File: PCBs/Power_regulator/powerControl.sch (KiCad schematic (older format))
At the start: 13 parts, among them J1 Conn_01x03_Female, J2 Conn_01x06_Female, J3 Conn_01x04_Male, J4 Conn_01x01_Male, J5 Conn_01x01_Male, J6 Conn_01x01_Male, J7 Conn_01x01_Male, J8 Conn_01x03_Female, J9 Conn_01x04_Female, U1 MAX9938

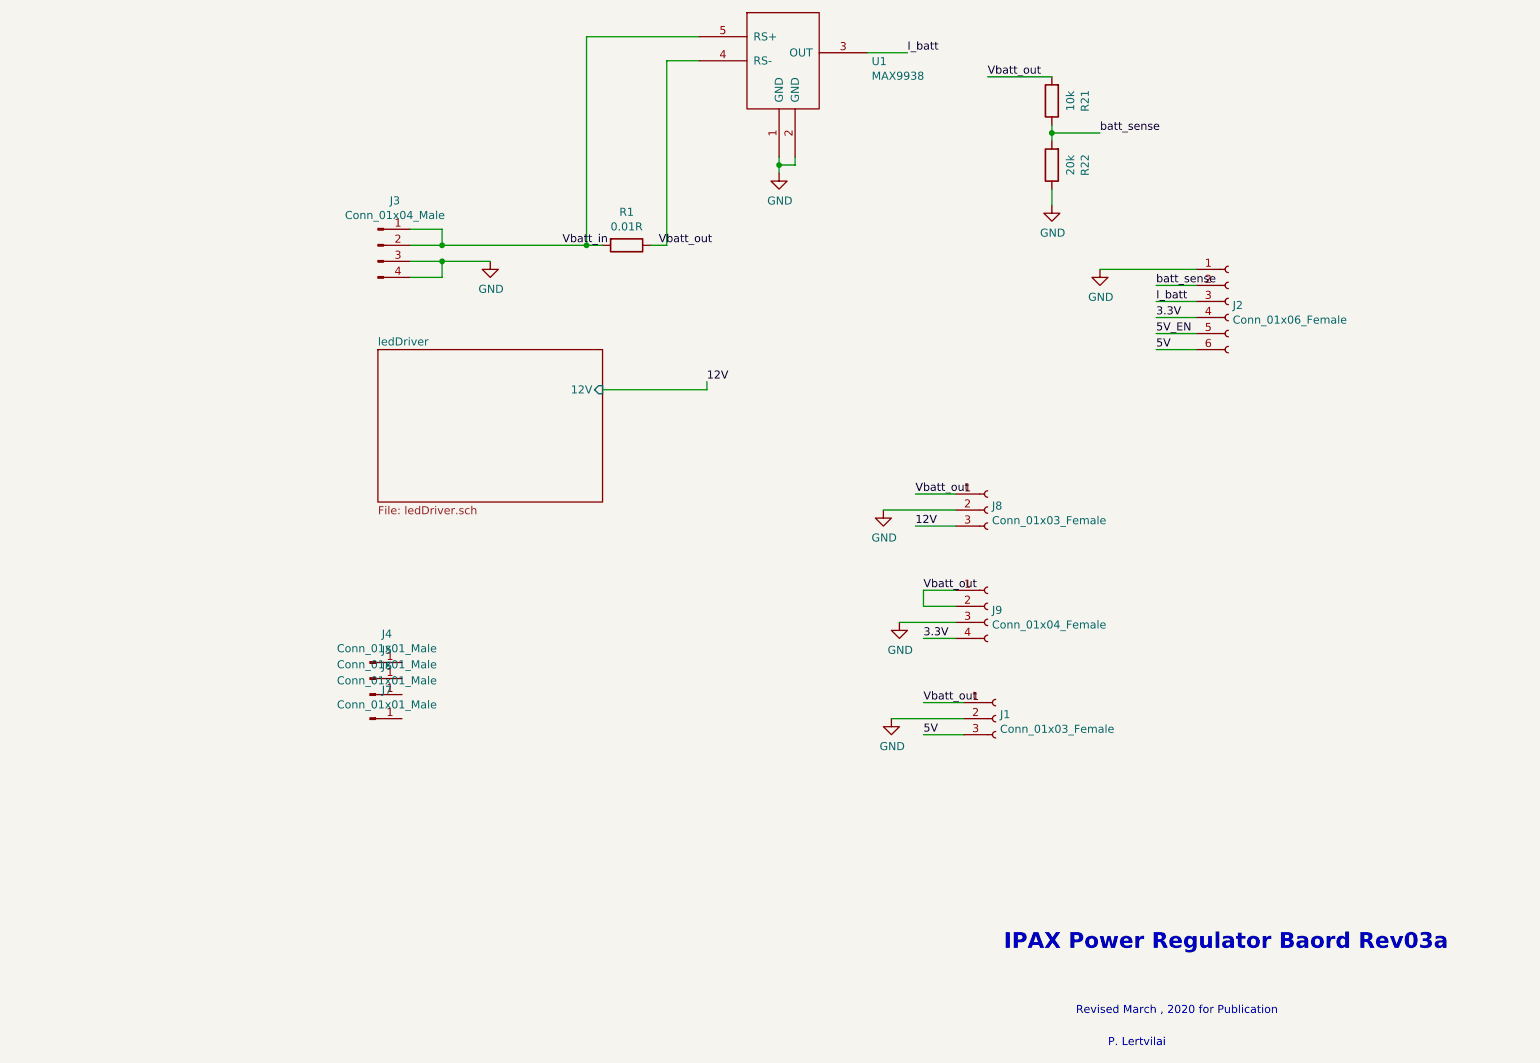
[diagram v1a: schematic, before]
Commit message: Update for revision05a
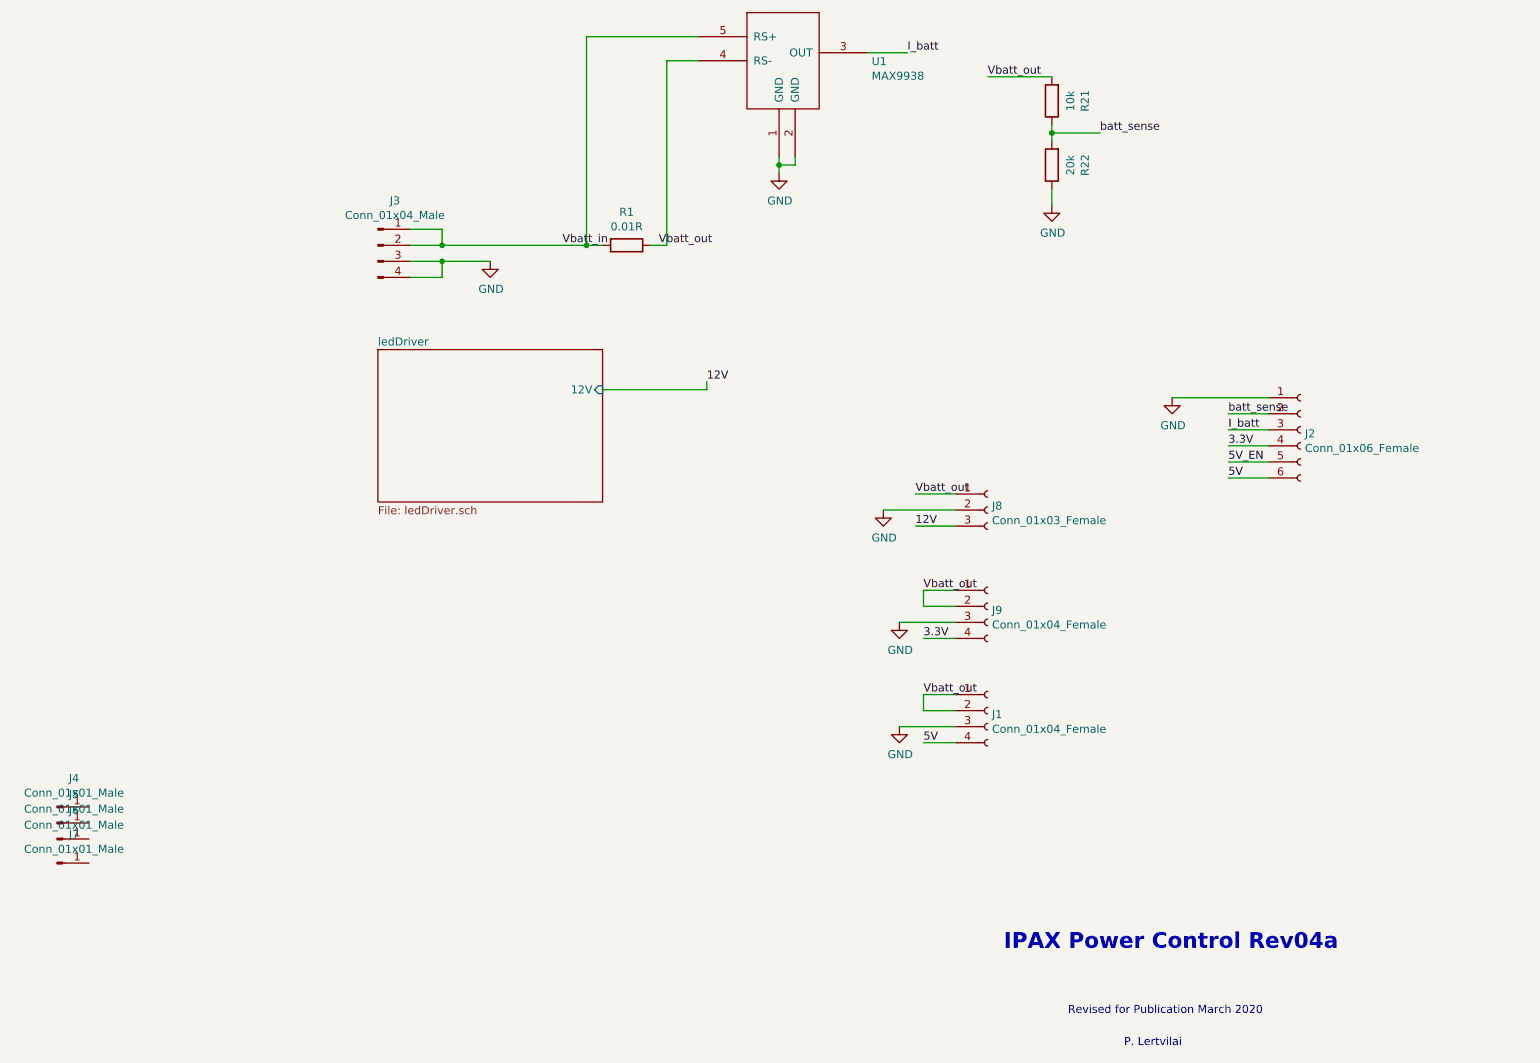
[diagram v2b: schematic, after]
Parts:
- removed J1: Conn_01x03_Female, Connector_PinHeader_2.54mm:PinHeader_1x03_P2.54mm_Vertical, symbol Connector:Conn_01x03_Female
- added J1: Conn_01x04_Female, Connector_PinHeader_2.54mm:PinHeader_1x04_P2.54mm_Vertical, symbol Connector:Conn_01x04_Female
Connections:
- net 5V: now also J1.4 (Pin_4)
- net GND: now also J1.3 (Pin_3)
- net Vbatt_out: now also J1.1 (Pin_1), J1.2 (Pin_2)
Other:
- note added: "IPAX Power Control Rev04a"
- note added: "Revised for Publication March 2020"
- note removed: "IPAX Power Regulator Baord Rev03a"
- note removed: "Revised March , 2020 for Publication"
- moved on the sheet: J2, J4, J5, J6, J7
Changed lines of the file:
@@
 L Connector:Conn_01x01_Male J4
 U 1 1 5C4AB1CA
-P 4200 5100
-F 0 "J4" H 4306 5278 50  0000 C CNN
-F 1 "Conn_01x01_Male" H 4306 5187 50  0000 C CNN
-F 2 "myLib:SCREW_4" H 4200 5100 50  0001 C CNN
-F 3 "~" H 4200 5100 50  0001 C CNN
-	1    4200 5100
+P 2250 6000
+F 0 "J4" H 2356 6178 50  0000 C CNN
+F 1 "Conn_01x01_Male" H 2356 6087 50  0000 C CNN
+F 2 "myLib:SCREW_4" H 2250 6000 50  0001 C CNN
+F 3 "~" H 2250 6000 50  0001 C CNN
+	1    2250 6000
 	1    0    0    -1
 $EndComp
@@
 L Connector:Conn_01x01_Male J5
 U 1 1 5C4AB288
-P 4200 5200
-F 0 "J5" H 4306 5378 50  0000 C CNN
-F 1 "Conn_01x01_Male" H 4306 5287 50  0000 C CNN
-F 2 "myLib:SCREW_4" H 4200 5200 50  0001 C CNN
-F 3 "~" H 4200 5200 50  0001 C CNN
-	1    4200 5200
+P 2250 6100
+F 0 "J5" H 2356 6278 50  0000 C CNN
+F 1 "Conn_01x01_Male" H 2356 6187 50  0000 C CNN
+F 2 "myLib:SCREW_4" H 2250 6100 50  0001 C CNN
+F 3 "~" H 2250 6100 50  0001 C CNN
+	1    2250 6100
 	1    0    0    -1
 $EndComp
@@
 L Connector:Conn_01x01_Male J6
 U 1 1 5C4AB2A4
-P 4200 5300
-F 0 "J6" H 4306 5478 50  0000 C CNN
-F 1 "Conn_01x01_Male" H 4306 5387 50  0000 C CNN
-F 2 "myLib:SCREW_4" H 4200 5300 50  0001 C CNN
-F 3 "~" H 4200 5300 50  0001 C CNN
-	1    4200 5300
+P 2250 6200
+F 0 "J6" H 2356 6378 50  0000 C CNN
+F 1 "Conn_01x01_Male" H 2356 6287 50  0000 C CNN
+F 2 "myLib:SCREW_4" H 2250 6200 50  0001 C CNN
+F 3 "~" H 2250 6200 50  0001 C CNN
+	1    2250 6200
 	1    0    0    -1
 $EndComp
@@
 L Connector:Conn_01x01_Male J7
 U 1 1 5C4AB2C4
-P 4200 5450
-F 0 "J7" H 4306 5628 50  0000 C CNN
-F 1 "Conn_01x01_Male" H 4306 5537 50  0000 C CNN
-F 2 "myLib:SCREW_4" H 4200 5450 50  0001 C CNN
-F 3 "~" H 4200 5450 50  0001 C CNN
-	1    4200 5450
+P 2250 6350
+F 0 "J7" H 2356 6528 50  0000 C CNN
+F 1 "Conn_01x01_Male" H 2356 6437 50  0000 C CNN
+F 2 "myLib:SCREW_4" H 2250 6350 50  0001 C CNN
+F 3 "~" H 2250 6350 50  0001 C CNN
+	1    2250 6350
 	1    0    0    -1
 $EndComp
@@
 L Connector:Conn_01x06_Female J2
 U 1 1 5C3E1CC8
-P 9550 2850
-F 0 "J2" H 9577 2826 50  0000 L CNN
-F 1 "Conn_01x06_Female" H 9577 2735 50  0000 L CNN
-F 2 "myLib:conn_1x06_1.5mm" H 9550 2850 50  0001 C CNN
-F 3 "~" H 9550 2850 50  0001 C CNN
-	1    9550 2850
-	1    0    0    -1
-$EndComp
-Wire Wire Line
-	9350 2750 9100 2750
-Wire Wire Line
-	9350 2950 9100 2950
-Wire Wire Line
-	9100 2850 9350 2850
+P 10000 3650
+F 0 "J2" H 10027 3626 50  0000 L CNN
+F 1 "Conn_01x06_Female" H 10027 3535 50  0000 L CNN
+F 2 "myLib:conn_1x06_1.5mm" H 10000 3650 50  0001 C CNN
+F 3 "~" H 10000 3650 50  0001 C CNN
+	1    10000 3650
+	1    0    0    -1
+$EndComp
+Wire Wire Line
+	9800 3550 9550 3550
+Wire Wire Line
+	9800 3750 9550 3750
+Wire Wire Line
+	9550 3650 9800 3650
 $Comp
 L power:GND #PWR0104
 U 1 1 5C459C2E
-P 8750 2650
-F 0 "#PWR0104" H 8750 2400 50  0001 C CNN
-F 1 "GND" H 8755 2477 50  0000 C CNN
-F 2 "" H 8750 2650 50  0001 C CNN
-F 3 "" H 8750 2650 50  0001 C CNN
-	1    8750 2650
-	1    0    0    -1
-$EndComp
-Text Label 9100 3150 0    50   ~ 0
+P 9200 3450
+F 0 "#PWR0104" H 9200 3200 50  0001 C CNN
+F 1 "GND" H 9205 3277 50  0000 C CNN
+F 2 "" H 9200 3450 50  0001 C CNN
+F 3 "" H 9200 3450 50  0001 C CNN
+	1    9200 3450
+	1    0    0    -1
+$EndComp
+Text Label 9550 3950 0    50   ~ 0
 5V
-Text Label 9100 2950 0    50   ~ 0
+Text Label 9550 3750 0    50   ~ 0
 3.3V
-Text Label 9100 3050 0    50   ~ 0
+Text Label 9550 3850 0    50   ~ 0
 5V_EN
 Wire Wire Line
-	8750 2650 9350 2650
+	9200 3450 9800 3450
 Text Notes 8150 6900 0    98   ~ 20
-IPAX Power Regulator Baord Rev03a
+IPAX Power Control Rev04a
 $Comp
 L Device:R R21
@@
 	-1   0    0    1
 $EndComp
-$Comp
-L Connector:Conn_01x03_Female J1
-U 1 1 5C4E6BD5
-P 8100 5450
-F 0 "J1" H 8127 5476 50  0000 L CNN
-F 1 "Conn_01x03_Female" H 8127 5385 50  0000 L CNN
-F 2 "Connector_PinHeader_2.54mm:PinHeader_1x03_P2.54mm_Vertical" H 8100 5450 50  0001 C CNN
-F 3 "~" H 8100 5450 50  0001 C CNN
-	1    8100 5450
-	1    0    0    -1
-$EndComp
 Wire Wire Line
 	8450 1450 8050 1450
@@
 Text Label 7550 1300 0    50   ~ 0
 I_batt
-$Comp
-L power:GND #PWR0105
-U 1 1 5C495E50
-P 7450 5450
-F 0 "#PWR0105" H 7450 5200 50  0001 C CNN
-F 1 "GND" H 7455 5277 50  0000 C CNN
-F 2 "" H 7450 5450 50  0001 C CNN
-F 3 "" H 7450 5450 50  0001 C CNN
-	1    7450 5450
-	1    0    0    -1
-$EndComp
-Wire Wire Line
-	9350 3050 9100 3050
-Wire Wire Line
-	9350 3150 9100 3150
-Text Label 9100 2850 0    50   ~ 0
+Wire Wire Line
+	9800 3850 9550 3850
+Wire Wire Line
+	9800 3950 9550 3950
+Text Label 9550 3650 0    50   ~ 0
 I_batt
-Text Label 9100 2750 0    50   ~ 0
+Text Label 9550 3550 0    50   ~ 0
 batt_sense
 $Comp
@@
 	4950 2600 4650 2600
 Connection ~ 4650 2600
-Wire Wire Line
-	7900 5350 7650 5350
-Wire Wire Line
-	7900 5450 7450 5450
-Wire Wire Line
-	7900 5550 7650 5550
-Text Label 7650 5350 0    50   ~ 0
-Vbatt_out
-Text Label 7650 5550 0    50   ~ 0
-5V
 $Comp
 L Connector:Conn_01x03_Female J8
@@
 Text Label 6300 3350 0    50   ~ 0
 12V
-Text Notes 8600 7300 0    50   ~ 0
-Revised March , 2020 for Publication
-Text Notes 8800 7500 0    50   ~ 0
+Text Notes 8550 7300 0    50   ~ 0
+Revised for Publication March 2020
+Text Notes 8900 7500 0    50   ~ 0
 P. Lertvilai
+$Comp
+L Connector:Conn_01x04_Female J1
+U 1 1 5E68AE60
+P 8050 5400
+F 0 "J1" H 8077 5376 50  0000 L CNN
+F 1 "Conn_01x04_Female" H 8077 5285 50  0000 L CNN
+F 2 "Connector_PinHeader_2.54mm:PinHeader_1x04_P2.54mm_Vertical" H 8050 5400 50  0001 C CNN
+F 3 "~" H 8050 5400 50  0001 C CNN
+	1    8050 5400
+	1    0    0    -1
+$EndComp
+Wire Wire Line
+	7850 5300 7650 5300
+Wire Wire Line
+	7650 5300 7650 5400
+Wire Wire Line
+	7650 5400 7850 5400
+Text Label 7650 5300 0    50   ~ 0
+Vbatt_out
+$Comp
+L power:GND #PWR0105
+U 1 1 5E68AE6A
+P 7500 5500
+F 0 "#PWR0105" H 7500 5250 50  0001 C CNN
+F 1 "GND" H 7505 5327 50  0000 C CNN
+F 2 "" H 7500 5500 50  0001 C CNN
+F 3 "" H 7500 5500 50  0001 C CNN
+	1    7500 5500
+	1    0    0    -1
+$EndComp
+Wire Wire Line
+	7850 5500 7500 5500
+Wire Wire Line
+	7850 5600 7650 5600
+Text Label 7650 5600 0    50   ~ 0
+5V
 $EndSCHEMATC
